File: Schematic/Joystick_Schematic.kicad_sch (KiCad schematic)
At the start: 16 parts, among them SW1 RKJXT1F42001, SW2 SKQUCAA010, SW3 SKQUCAA010, SW4 SKQUCAA010, SW5 SKQUCAA010, U2 SeeeduinoXIAO

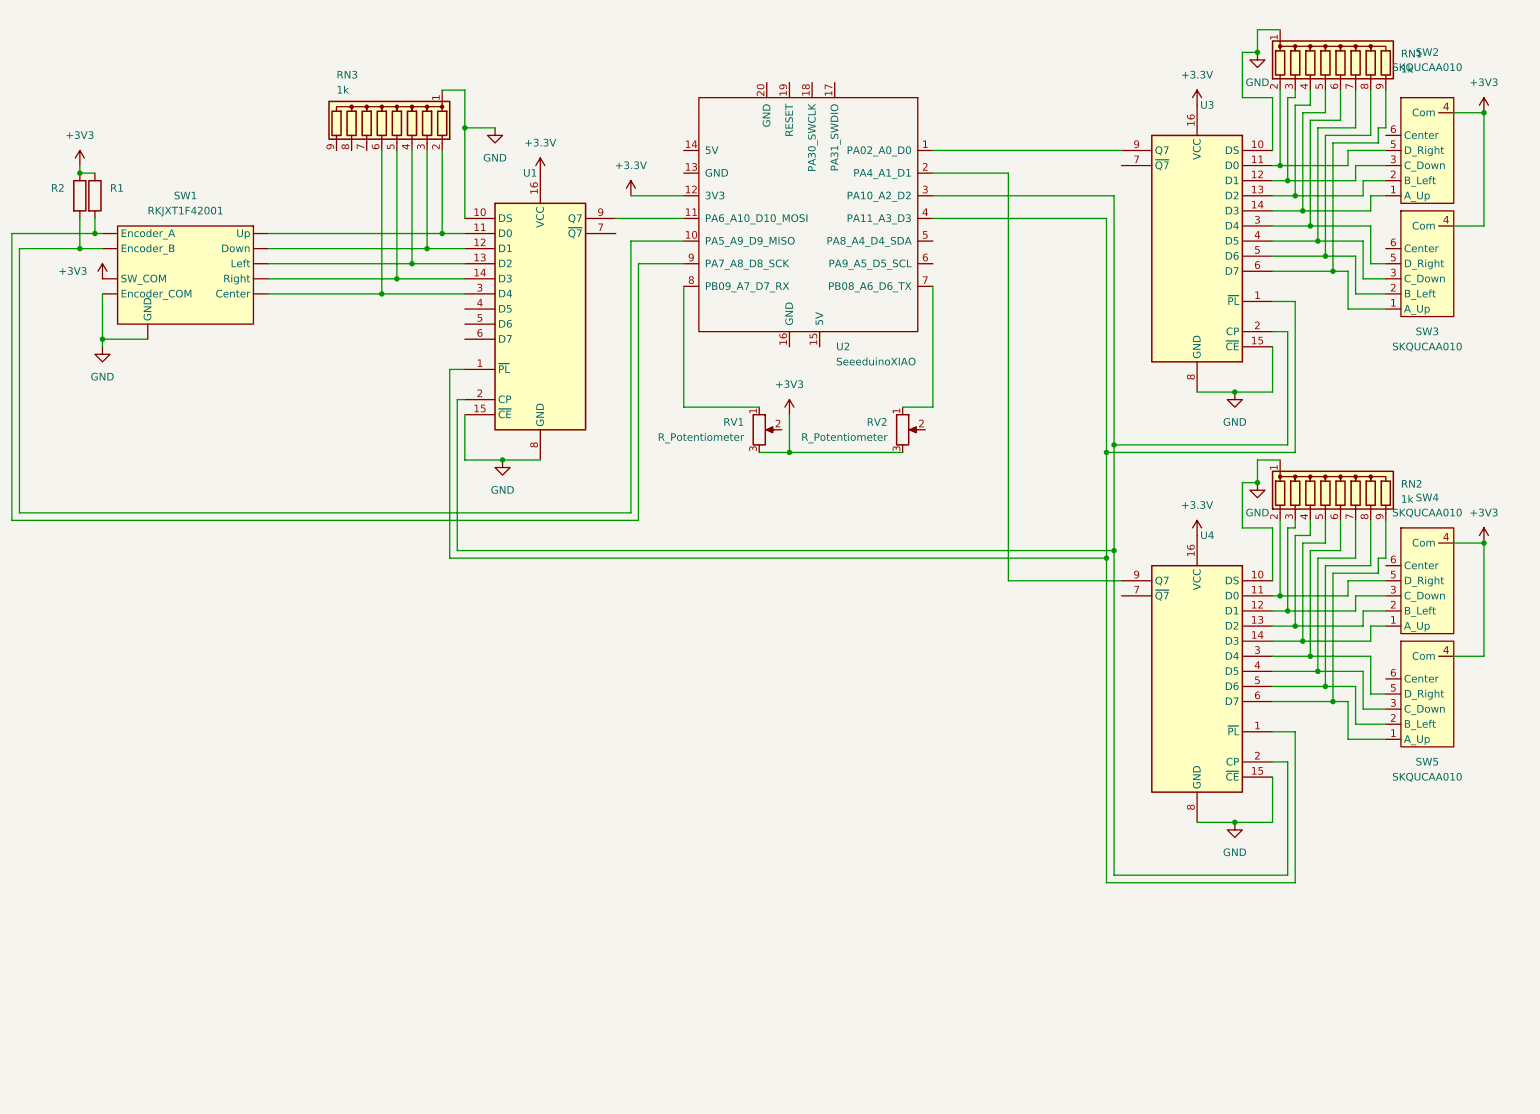
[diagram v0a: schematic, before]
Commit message: Schematic update again and started PCB
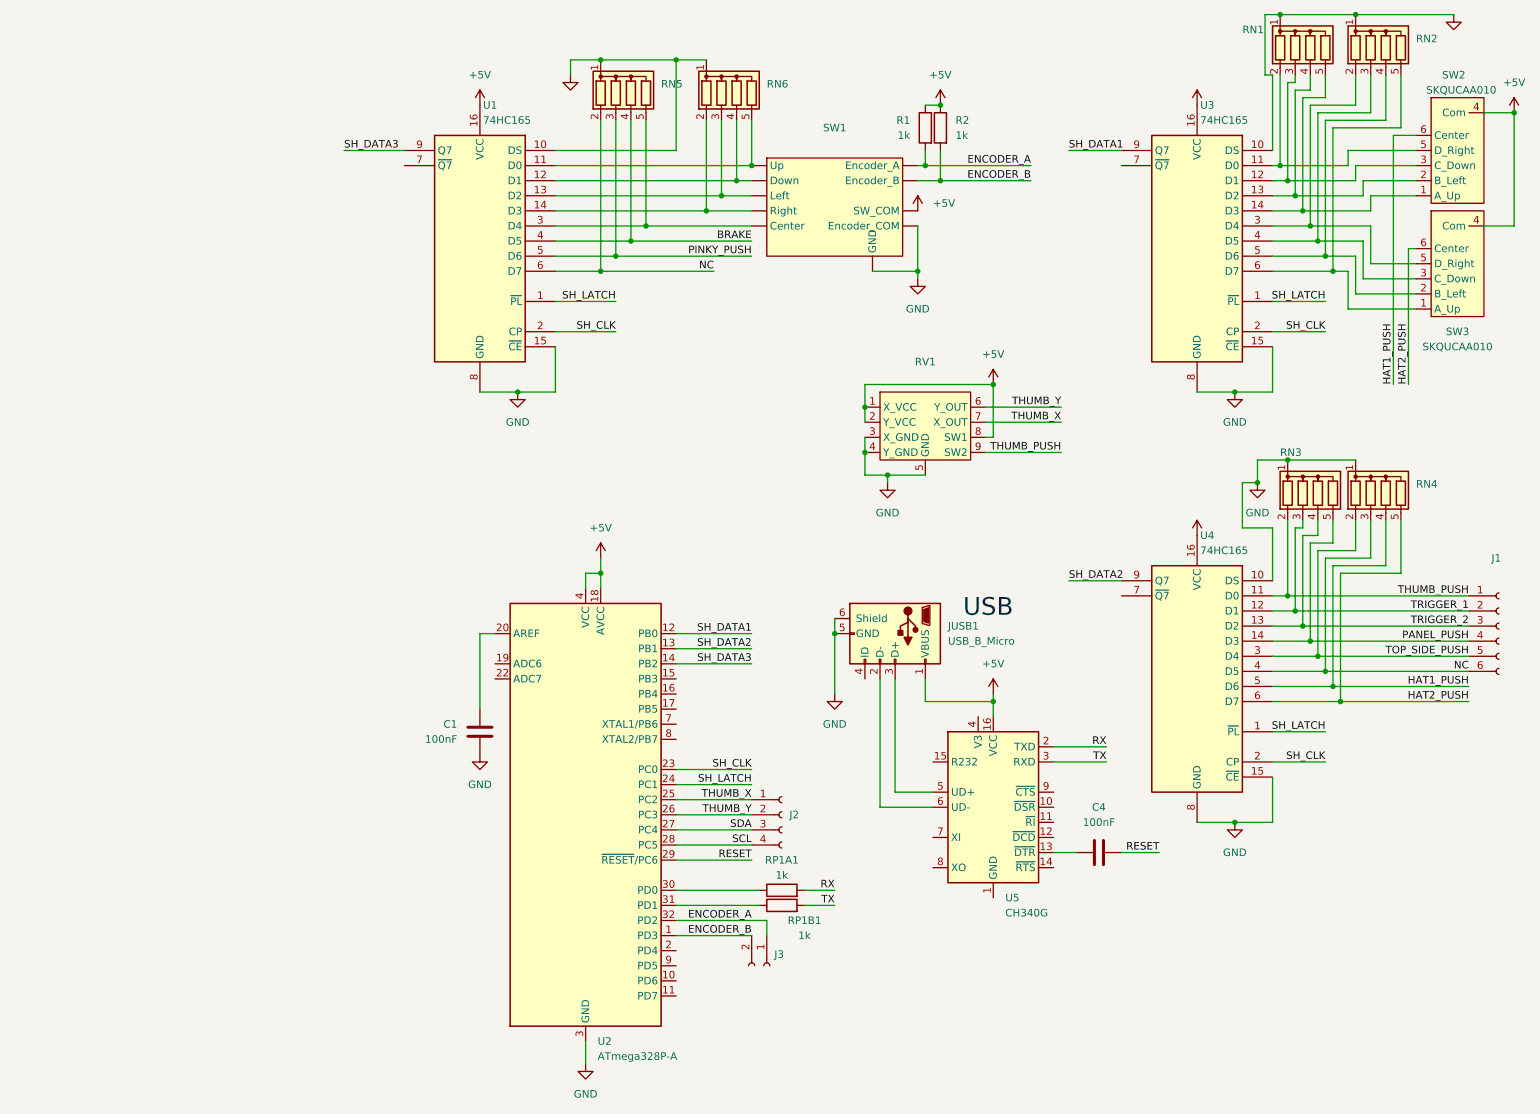
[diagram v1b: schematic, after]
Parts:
- removed RN1, RN2, RN3: 1k, Resistor_THT:R_Array_SIP9, symbol Device:R_Network08
- removed RV1, RV2: R_Potentiometer, symbol Device:R_Potentiometer
- removed SW4, SW5: SKQUCAA010, Alps-SKQU:SKQUCAA010, symbol Alps-SKQU:SKQUCAA010
- removed U2: SeeeduinoXIAO, Seeeduino XIAO KICAD:Seeeduino XIAO-MOUDLE14P-2.54-21X17.8MM, symbol Seeeduino XIAO:SeeeduinoXIAO
- added C1, C4: 100nF, Resistor_SMD:R_0201_0603Metric_Pad0.64x0.40mm_HandSolder, symbol Device:C
- added J1: (no value), symbol Connector:Conn_01x06_Female
- added J2: (no value), symbol Connector:Conn_01x04_Female
- added J3: (no value), symbol Connector:Conn_01x02_Female
- added JUSB1: USB_B_Micro, Connector_USB:USB_Micro-B_Molex_47346-0001, symbol Connector:USB_B_Micro
- added RN1, RN2, RN3, RN4, RN5, RN6: (no value), symbol Device:R_Network04
- added RP1A1, RP1B1: 1k, Resistor_SMD:R_0201_0603Metric_Pad0.64x0.40mm_HandSolder, symbol Device:R
- added RV1: (no value), symbol Alps-RKJXV:RKJXV122400R
- added U2: ATmega328P-A, Package_QFP:TQFP-32_7x7mm_P0.8mm, symbol MCU_Microchip_ATmega:ATmega328P-A
- added U5: CH340G, Package_SO:SOIC-16_3.9x9.9mm_P1.27mm, symbol Interface_USB:CH340G
- R1, R2: value (none) -> 1k; footprint (none) -> Resistor_SMD:R_0201_0603Metric_Pad0.64x0.40mm_HandSolder
- SW1: value RKJXT1F42001 -> (none)
- U1, U3, U4: value (none) -> 74HC165; footprint (none) -> Package_SO:TSSOP-16_4.4x5mm_P0.65mm
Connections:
- net GND: now also C1.2, JUSB1.5 (GND), JUSB1.6 (Shield), RN1.1 (common), RN2.1 (common), RN3.1 (common), RN4.1 (common), RN5.1 (common), RN6.1 (common), RV1.3 (X_GND), RV1.4 (Y_GND), RV1.5 (GND), U2.21 (GND), U2.3 (GND), U2.5 (GND)
- net SH_DATA1: now reaches U3.9 (Q7)
- net SH_DATA1: now also U2.12 (PB0)
- net ENCODER_B: now reaches R2.2, SW1. (Up)
- net ENCODER_B: now also J3.2 (Pin_2), U2.1 (PD3)
- net SH_DATA3: now reaches U1.9 (Q7)
- net SH_DATA3: now also U2.14 (PB2)
- net SH_DATA2: now reaches U4.9 (Q7)
- net SH_DATA2: now also U2.13 (PB1)
- net SH_CLK: now reaches U1.2 (CP), U3.2 (CP), U4.2 (CP)
- net SH_CLK: now also U2.23 (PC0)
- net SH_LATCH: now reaches U1.1 (~{PL}), U3.1 (~{PL}), U4.1 (~{PL})
- net SH_LATCH: now also U2.24 (PC1)
- net ENCODER_A: now reaches R1.2, SW1. (Up)
- net ENCODER_A: now also J3.1 (Pin_1), U2.32 (PD2)
- net at SW2.5 (D_Right), U3.11 (D0): now also RN1.2 (R1)
- net at SW2.3 (C_Down), U3.12 (D1): now also RN1.3 (R2)
- net at SW2.2 (B_Left), U3.13 (D2): now also RN1.4 (R3)
- net at SW2.1 (A_Up), U3.14 (D3): now also RN1.5 (R4)
- net at SW3.5 (D_Right), U3.3 (D4): now also RN2.2 (R1)
- net at SW3.3 (C_Down), U3.4 (D5): now also RN2.3 (R2)
- net at SW3.2 (B_Left), U3.5 (D6): now also RN2.4 (R3)
- net at SW3.1 (A_Up), U3.6 (D7): now also RN2.5 (R4)
- net HAT1_PUSH: now reaches SW2.6 (Center)
- net HAT1_PUSH: now also U4.5 (D6), RN4.4 (R3)
- net HAT2_PUSH: now reaches U4.6 (D7)
- net HAT2_PUSH: now also SW3.6 (Center), RN4.5 (R4)
- net NC: now reaches U4.4 (D5)
- net NC: now also U1.6 (D7), J1.6 (Pin_6), RN4.3 (R2), RN5.2 (R1)
- net TOP_SIDE_PUSH: now reaches U4.3 (D4)
- net TOP_SIDE_PUSH: now also J1.5 (Pin_5), RN4.2 (R1)
- net PANEL_PUSH: now reaches U4.14 (D3)
- net PANEL_PUSH: now also J1.4 (Pin_4), RN3.5 (R4)
- net TRIGGER_2: now reaches U4.13 (D2)
- net TRIGGER_2: now also J1.3 (Pin_3), RN3.4 (R3)
- net TRIGGER_1: now reaches U4.12 (D1)
- net TRIGGER_1: now also J1.2 (Pin_2), RN3.3 (R2)
- net THUMB_PUSH: now reaches U4.11 (D0)
- net THUMB_PUSH: now also J1.1 (Pin_1), RN3.2 (R1), RV1.9 (SW2)
- net at SW1. (Up), U1.11 (D0): now also RN6.5 (R4)
- net at SW1. (Up), U1.12 (D1): now also RN6.4 (R3)
- net at SW1. (Up), U1.13 (D2): now also RN6.3 (R2)
- net at SW1. (Up), U1.14 (D3): now also RN6.2 (R1)
- net at SW1. (Up), U1.3 (D4): now also RN5.5 (R4)
- net BRAKE: now reaches U1.4 (D5)
- net BRAKE: now also RN5.4 (R3)
- net PINKY_PUSH: now reaches U1.5 (D6)
- net PINKY_PUSH: now also RN5.3 (R2)
- net +3V3 renamed +5V
- net +5V: now also JUSB1.1 (VBUS), RV1.1 (X_VCC), RV1.2 (Y_VCC), RV1.8 (SW1), U2.18 (AVCC), U2.4 (VCC), U2.6 (VCC), U5.16 (VCC)
- new net: RP1B1.1, U2.31 (PD1)
- new net: C1.1, U2.20 (AREF)
- new net: RP1A1.1, U2.30 (PD0)
- new net: C4.1, U5.13 (~{DTR})
- new net: JUSB1.3 (D+), U5.5 (UD+)
- new net: JUSB1.2 (D-), U5.6 (UD-)
- new net RESET: C4.2, U2.29 (~{RESET}/PC6)
- new net RX: RP1A1.2, U5.2 (TXD)
- new net SCL: J2.4 (Pin_4), U2.28 (PC5)
- new net SDA: J2.3 (Pin_3), U2.27 (PC4)
- new net THUMB_X: J2.1 (Pin_1), RV1.7 (X_OUT), U2.25 (PC2)
- new net THUMB_Y: J2.2 (Pin_2), RV1.6 (Y_OUT), U2.26 (PC3)
- new net TX: RP1B1.2, U5.3 (RXD)
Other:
- note added: "USB"
- moved on the sheet: R1, R2, SW1, SW2, SW3, U1
